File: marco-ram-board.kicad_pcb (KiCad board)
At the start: 4 copper layers, 160 x 100 mm, 186 parts, among them J201 PRG_USB, J202 MCU_RST, J203 MCU_BOOT0, J204 FT_TXD, J205 FT_RXD, J206 CONN_JTAG, J301 CONN_MCU_SERIAL, J302 CONN_EXT, J501 MCU_USB, J502 SD_Card, J503 CONN_DISP, J504 RJ45_Amphenol_RJMG1BD3B8K1ANR, J601 CONN_JACK_12V, J602 CONN_SCREW_12V, Q201 MMBT3906, Q601 DMP3037LSS, SW301 SW_RST, SW302 SW_BOOT0, SW501 BTN0, SW502 BTN1, SW503 BTN2, SW504 BTN3, SW601 PWR_SW, U201 FT2232HL, U301 STM32F765IITx, U401 IS42S86400D, U402 IS42S86400D, U403 IS42S86400D, U404 IS42S86400D, U405 IS42S86400D, U406 IS42S86400D, U407 IS42S86400D, U408 IS42S86400D, U501 KSZ8081RNA, U601 LM2576S-3.3, Y201 12MHz, Y301 25MHz

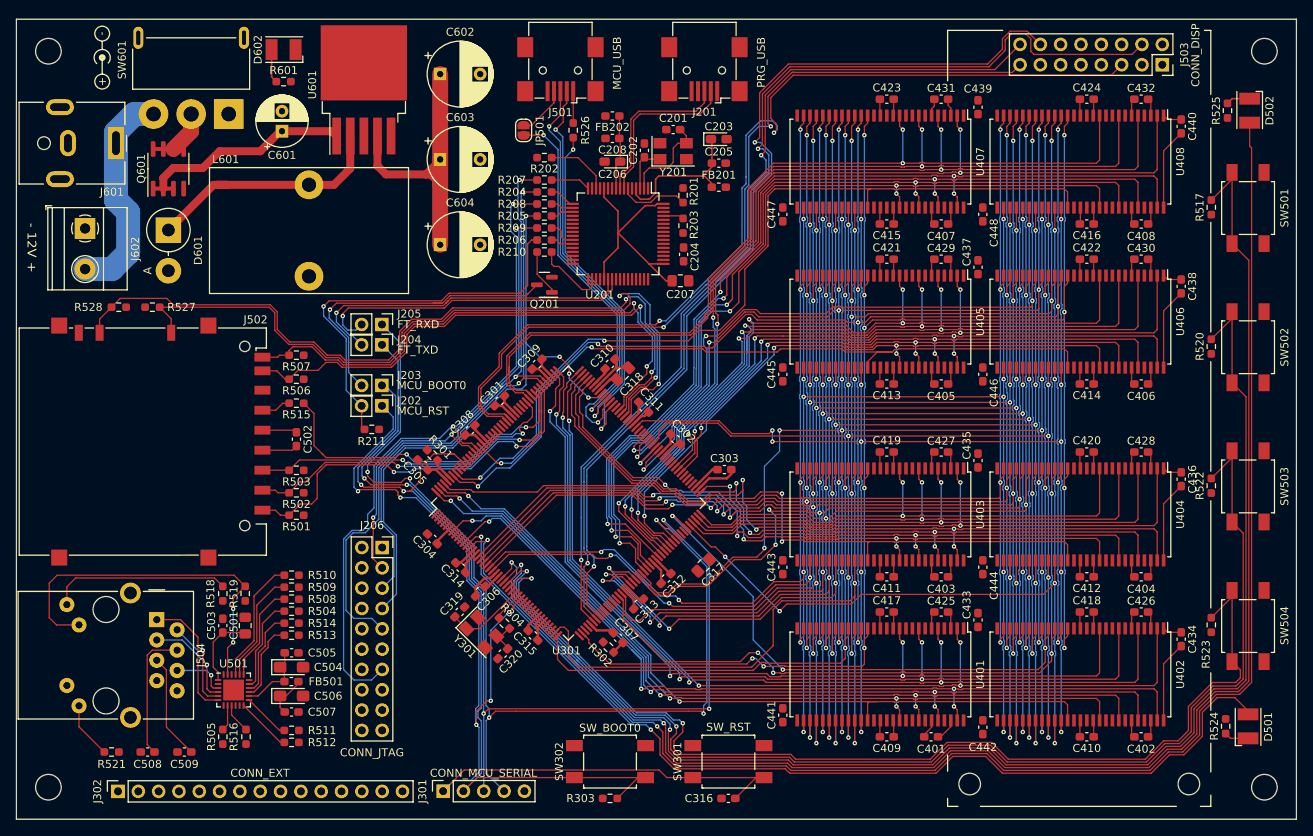
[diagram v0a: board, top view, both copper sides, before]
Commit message: Artwork cleanup
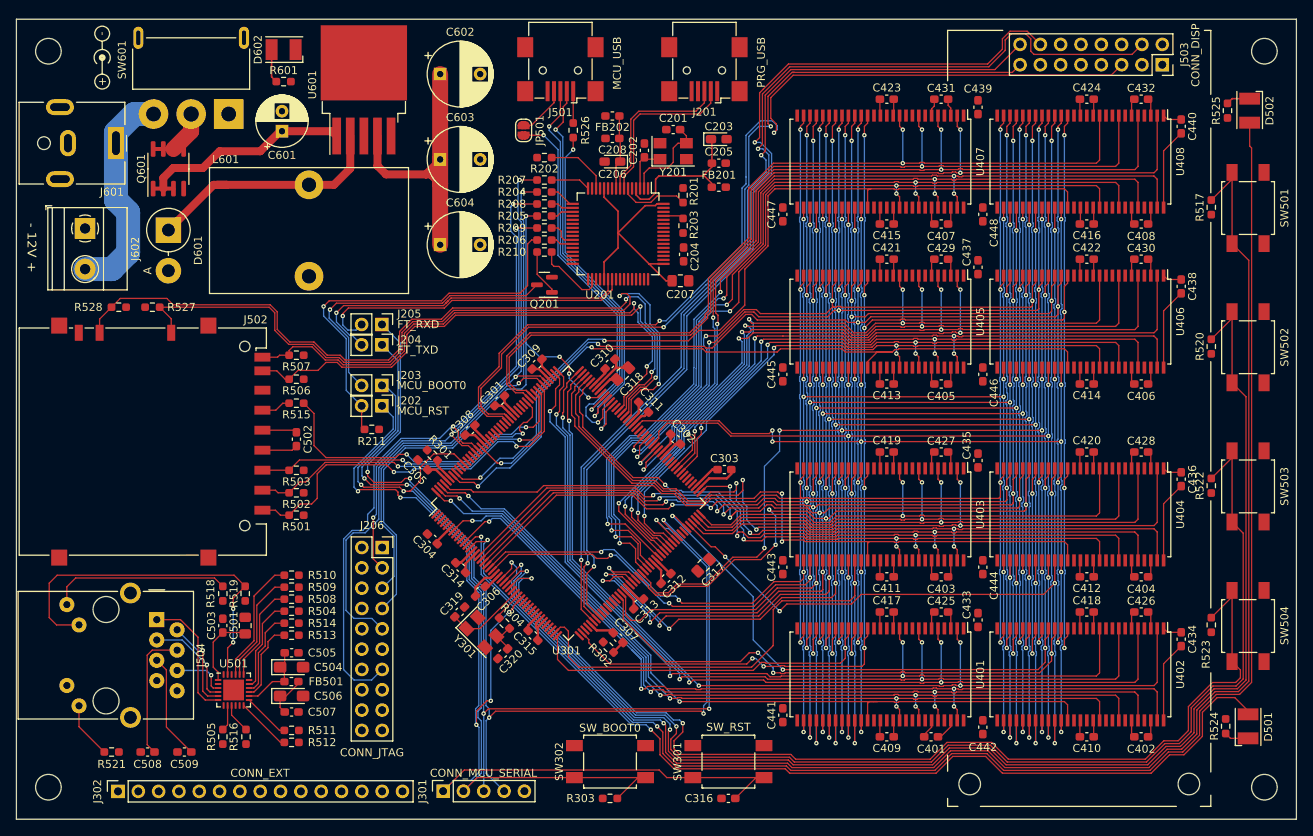
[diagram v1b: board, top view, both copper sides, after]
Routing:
- net VDD: track 170.7 -> 160.3 mm
- net GND: track 154.2 -> 147.1 mm
- net /mcu/SDRAM.D10: track 100.4 -> 98.3 mm
- net /mcu-if/DISP.MOSI: track 120.0 -> 118.4 mm
- net /mcu-if/SDMMC.D3: track 44.5 -> 43.3 mm
- net Net-(J203-Pad2): track 39.6 -> 38.3 mm
- net /mcu/SDRAM.D5: track 111.6 -> 110.8 mm
- net /mcu/SDRAM.D2: track 113.8 -> 113.0 mm
- net /mcu-if/SDMMC.D2: track 48.7 -> 48.0 mm
- net /mcu-if/SDMMC.CD: track 95.3 -> 94.7 mm
- net /mcu/BOOT0: track 103.0 -> 102.3 mm
- net /mcu-if/BTN0: track 187.2 -> 186.6 mm
